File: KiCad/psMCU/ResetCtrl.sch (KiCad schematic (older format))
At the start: 14 parts

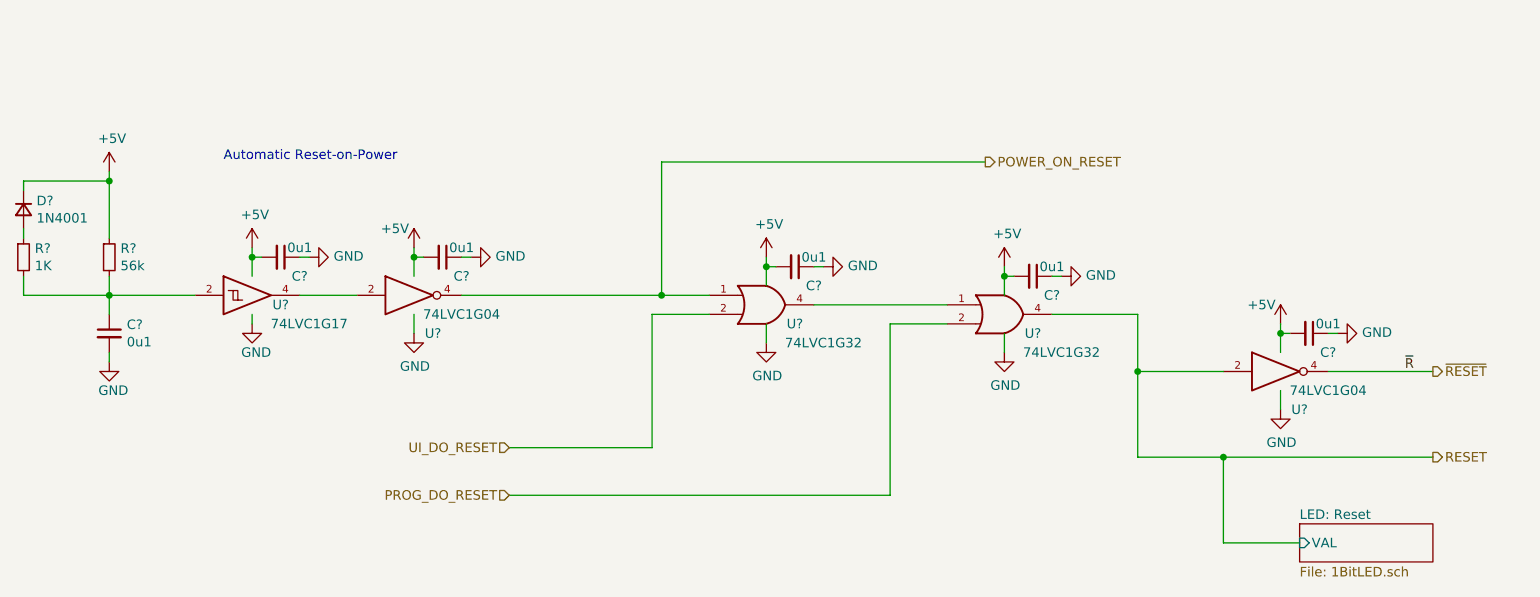
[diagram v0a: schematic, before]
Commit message: Started some documentation work.
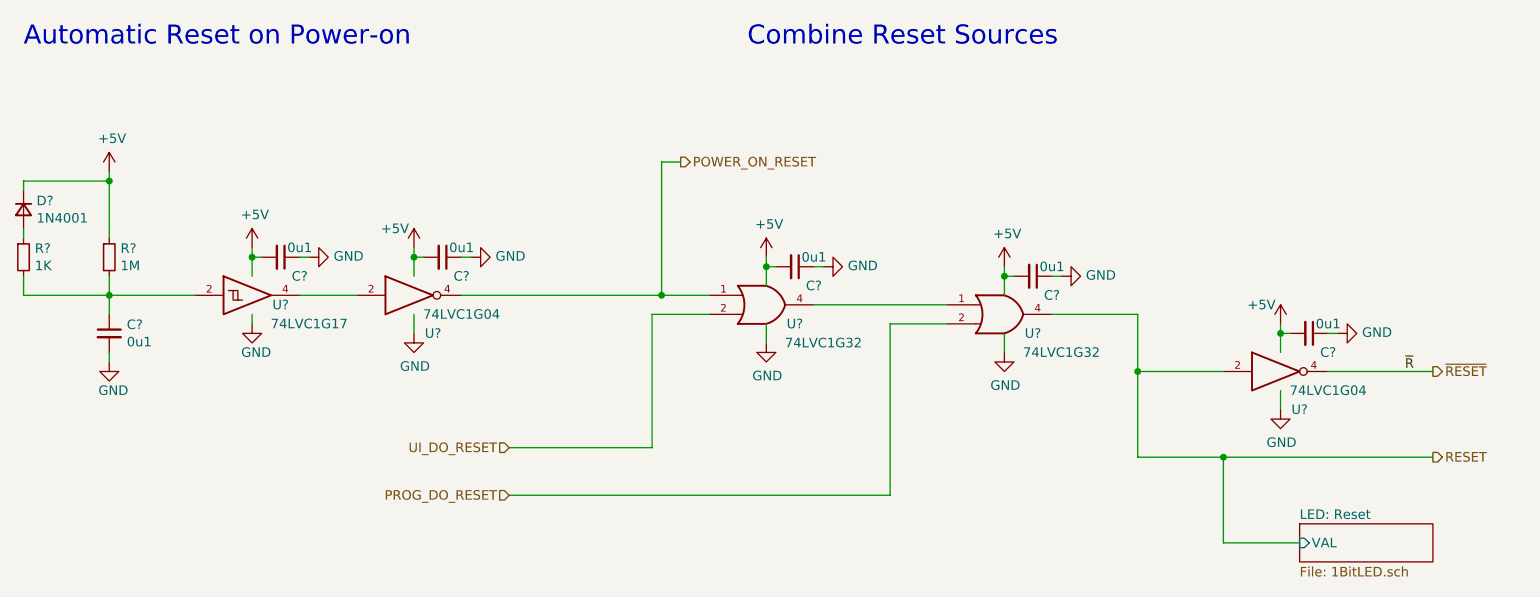
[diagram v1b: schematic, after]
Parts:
- R?: value 56k -> 1M
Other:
- note added: "Automatic Reset on Power-on"
- note added: "Combine Reset Sources"
- note removed: "Automatic Reset-on-Power"
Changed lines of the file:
@@
 Comment1 ""
 Comment2 ""
-Comment3 ""
-Comment4 ""
+Comment3 "generate the RESET and ~RESET~ signals used globally."
+Comment4 "Generates reset during power-on and combines the different reset sources to"
 $EndDescr
 Text Label 9250 3550 2    50   ~ 0
@@
 P 2400 2950
 F 0 "R?" H 2459 2996 50  0000 L CNN
-F 1 "56k" H 2459 2905 50  0000 L CNN
+F 1 "1M" H 2459 2905 50  0000 L CNN
 F 2 "Resistor_SMD:R_0603_1608Metric" H 2400 2950 50  0001 C CNN
 F 3 "~" H 2400 2950 50  0001 C CNN
@@
 Wire Wire Line
 	7800 3250 7800 3550
-Text Notes 3000 2450 0    50   ~ 0
-Automatic Reset-on-Power
-Text HLabel 7000 2450 2    50   Output ~ 0
+Text Notes 1950 1850 0    100  ~ 0
+Automatic Reset on Power-on
+Text HLabel 5400 2450 2    50   Output ~ 0
 POWER_ON_RESET
 Wire Wire Line
 	5300 2450 5300 3150
 Wire Wire Line
-	5300 2450 7000 2450
+	5300 2450 5400 2450
 Connection ~ 5300 3150
 Wire Wire Line
@@
 Wire Wire Line
 	8250 4000 7800 4000
+Text Notes 5750 1850 0    100  ~ 0
+Combine Reset Sources
 $EndSCHEMATC
